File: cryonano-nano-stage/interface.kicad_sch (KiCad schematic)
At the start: 24 parts, among them U7 LP5907MFX-3.3_NOPB, U8 LP5907MFX-3.3_NOPB

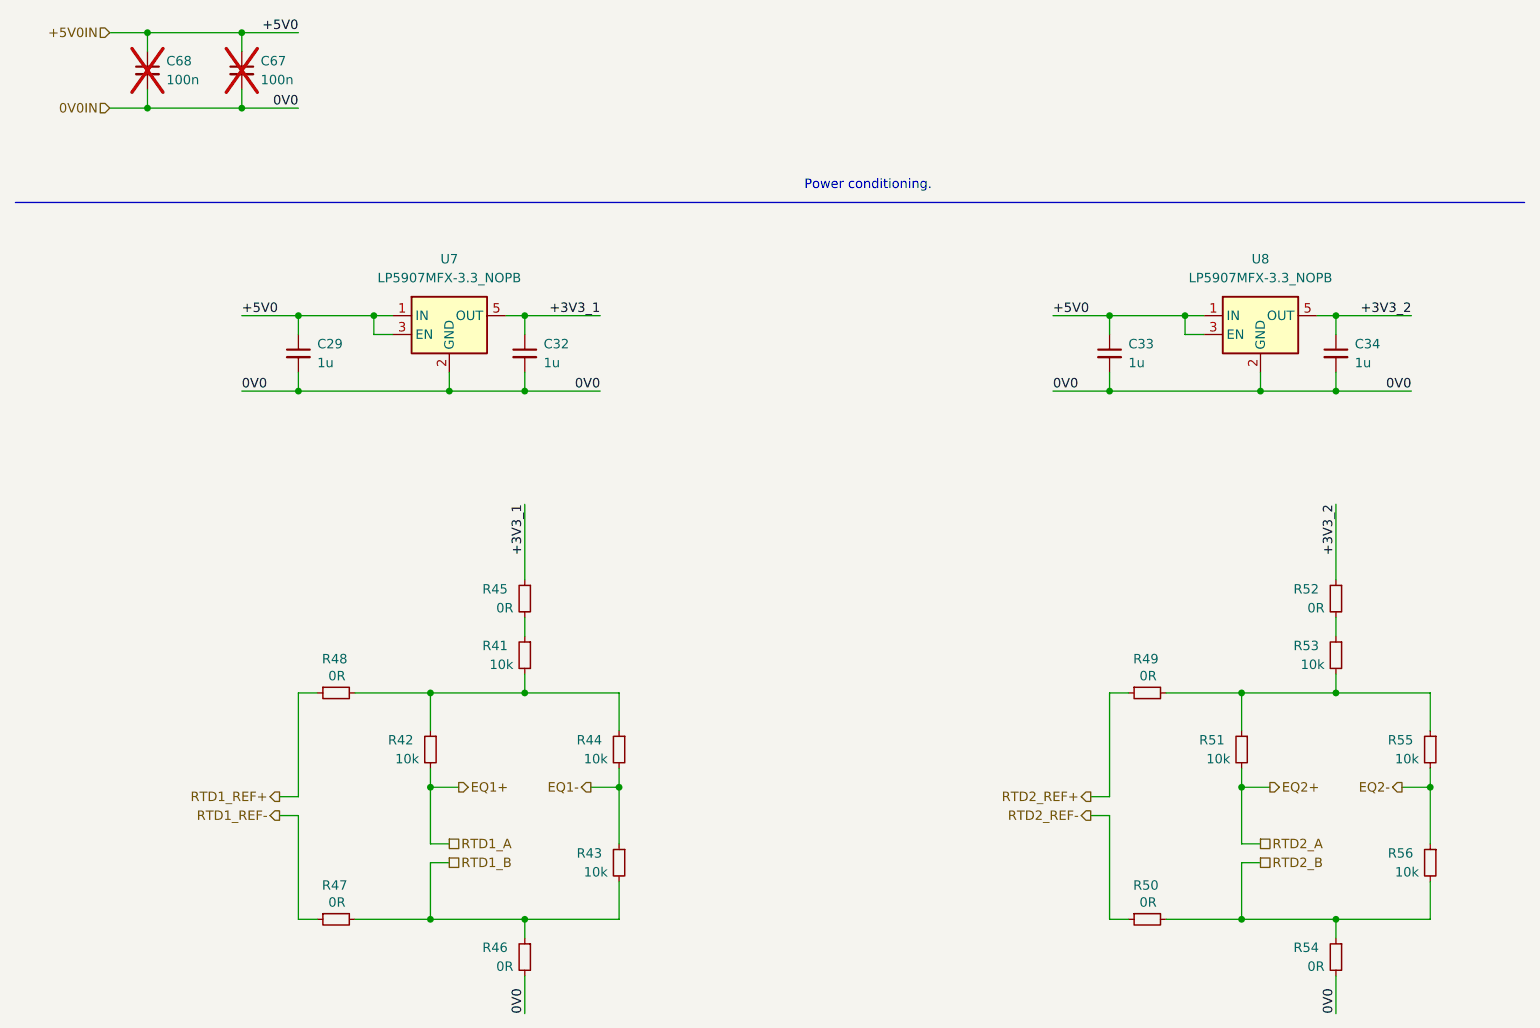
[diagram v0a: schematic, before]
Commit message: sch improved
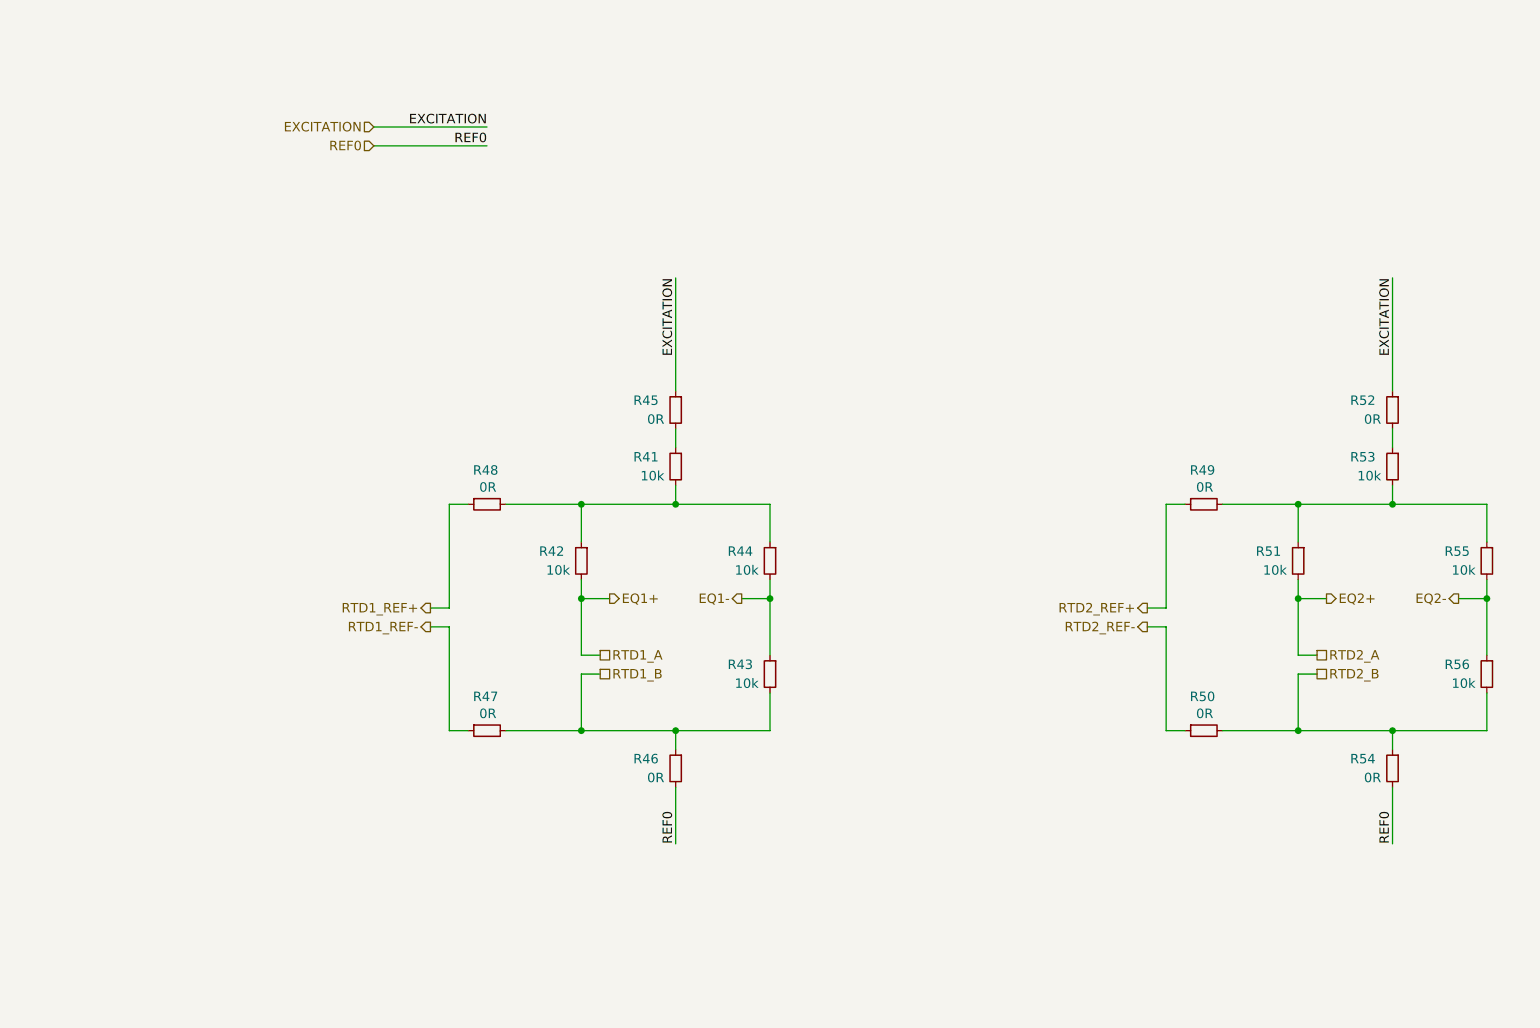
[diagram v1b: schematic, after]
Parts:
- removed C29, C32, C33, C34: 1u, Capacitor_SMD:C_0603_1608Metric, symbol Device:C_Small
- removed C67, C68: 100n, Capacitor_SMD:C_0603_1608Metric, symbol Device:C_Small
- removed U7, U8: LP5907MFX-3.3_NOPB, SOT95P280X145-5N, symbol symbols:LP5907MFX-3.3_NOPB
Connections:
- net +3V3_2 is gone; now on net EXCITATION: R52.1
- net +3V3_1 renamed EXCITATION
- net 0V0IN renamed REF0
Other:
- note removed: "Power conditioning."
- moved on the sheet: R41, R42, R43, R44, R45, R46, R47, R48, R49, R50, R51, R52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
